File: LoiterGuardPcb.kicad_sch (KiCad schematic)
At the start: 0 parts

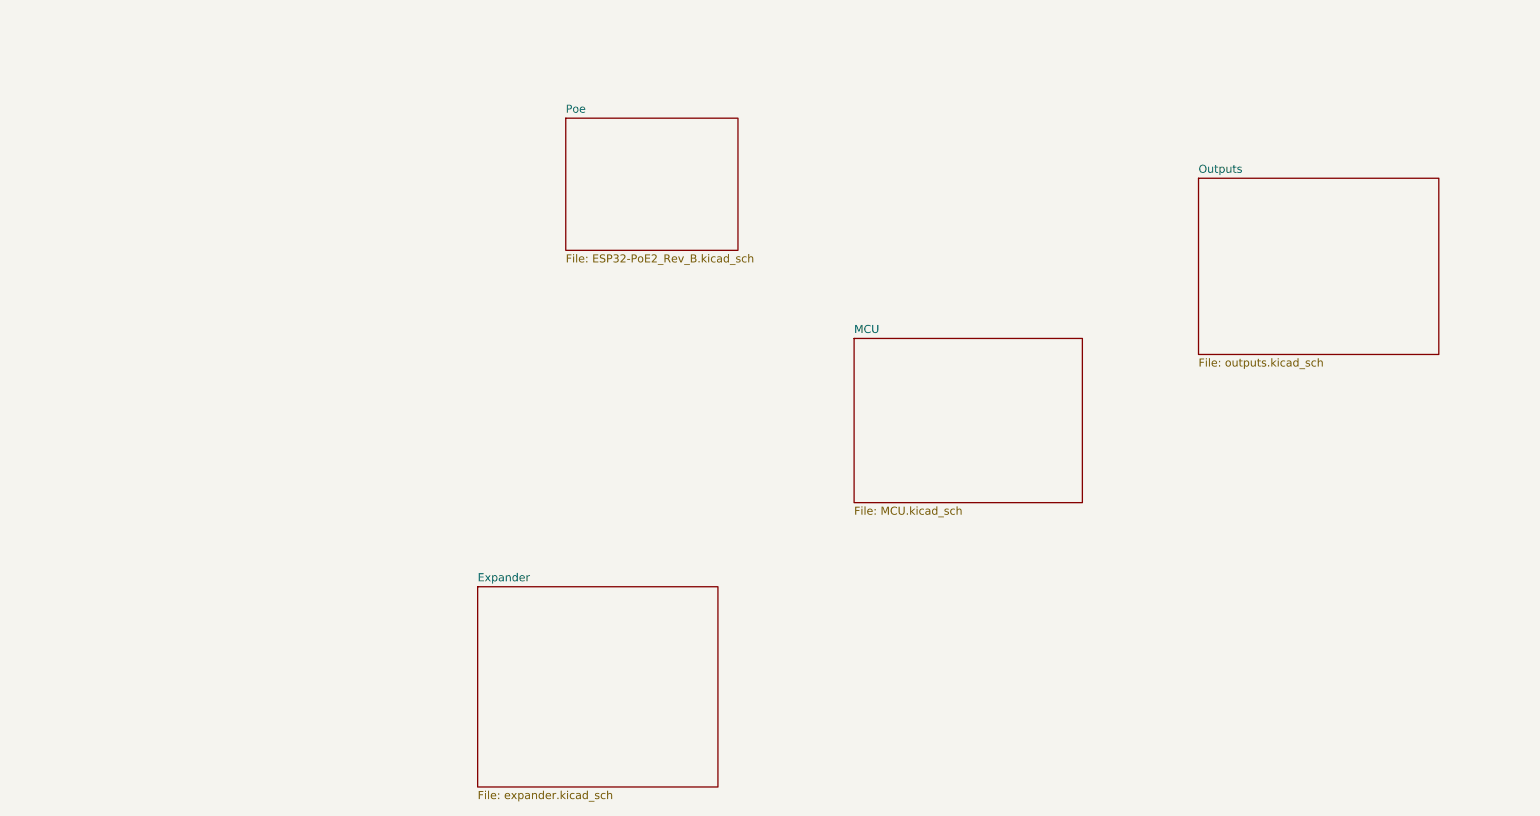
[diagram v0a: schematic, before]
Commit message: wip - started traces for layout
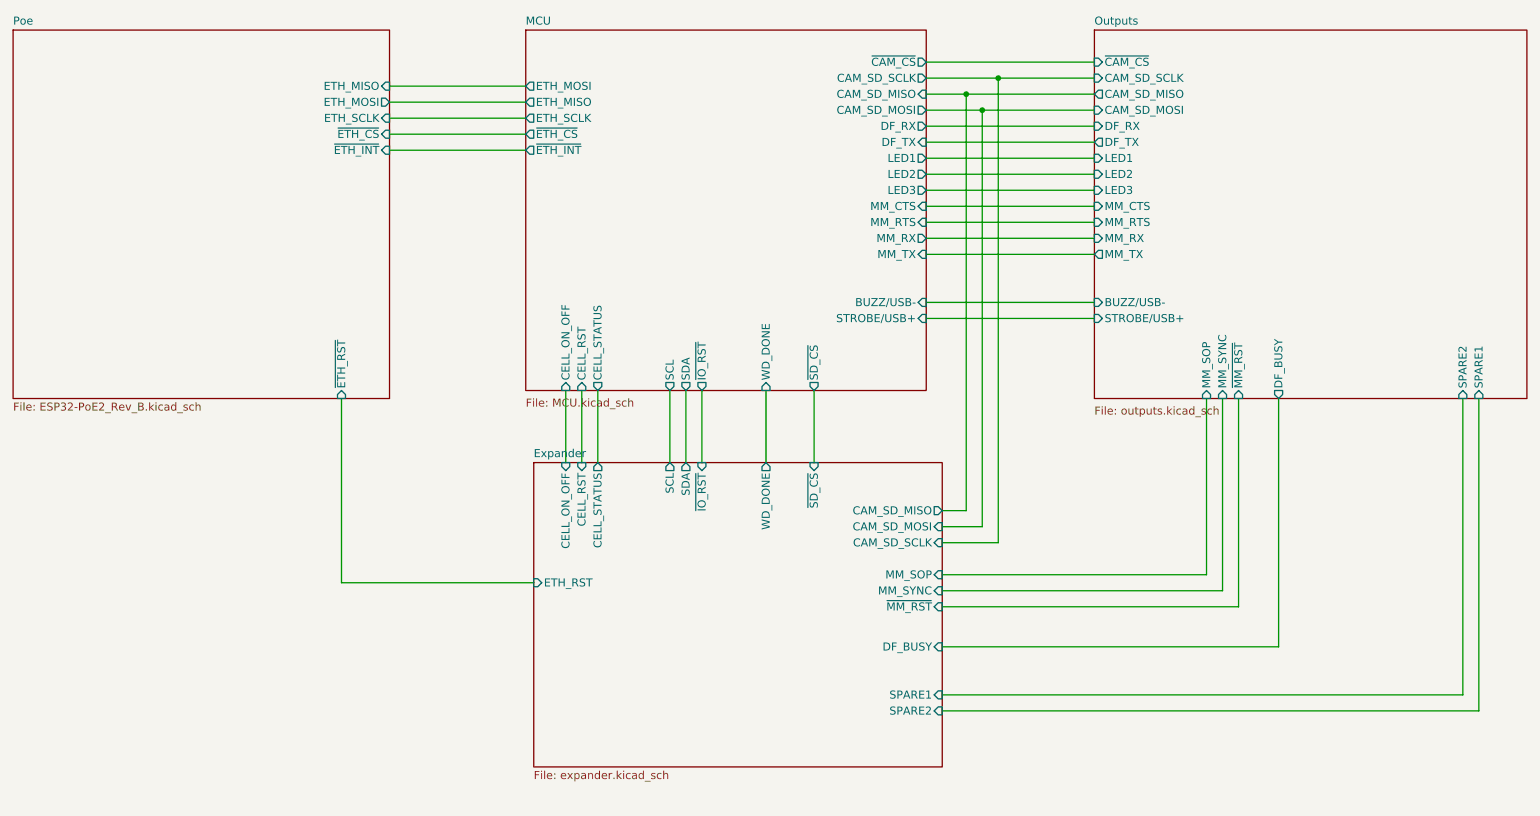
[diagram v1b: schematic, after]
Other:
- sheet Expander ports: added CAM_SD_MISO, CAM_SD_MOSI, CAM_SD_SCLK, CELL_ON_OFF, CELL_RST, CELL_STATUS, DF_BUSY, ETH_RST, MM_SOP, MM_SYNC, SCL, SDA, SPARE1, SPARE2, WD_DONE, ~{IO_RST}, ~{MM_RST}, ~{SD_CS}; removed none
- sheet MCU ports: added BUZZ/USB-, CAM_SD_MISO, CAM_SD_MOSI, CAM_SD_SCLK, CELL_ON_OFF, CELL_RST, CELL_STATUS, DF_RX, DF_TX, ETH_MISO, ETH_MOSI, ETH_SCLK, LED1, LED2, LED3, MM_CTS, MM_RTS, MM_RX, MM_TX, SCL, SDA, STROBE/USB+, WD_DONE, ~{CAM_CS}, ~{ETH_CS}, ~{ETH_INT}, ~{IO_RST}, ~{SD_CS}; removed none
- sheet Outputs ports: added BUZZ/USB-, CAM_SD_MISO, CAM_SD_MOSI, CAM_SD_SCLK, DF_BUSY, DF_RX, DF_TX, LED1, LED2, LED3, MM_CTS, MM_RTS, MM_RX, MM_SOP, MM_SYNC, MM_TX, SPARE1, SPARE2, STROBE/USB+, ~{CAM_CS}, ~{MM_RST}; removed none
- sheet Poe ports: added ETH_MISO, ETH_MOSI, ETH_SCLK, ~{ETH_CS}, ~{ETH_INT}, ~{ETH_RST}; removed none
